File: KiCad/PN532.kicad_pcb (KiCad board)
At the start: 2 copper layers, 40 x 40 mm, 56 parts, among them J1 Bell, J2 Header, J3 SPOX, SW1 TAMPER, U1 PN532, U2 QR, U3 QR, Y1 27.12MHz

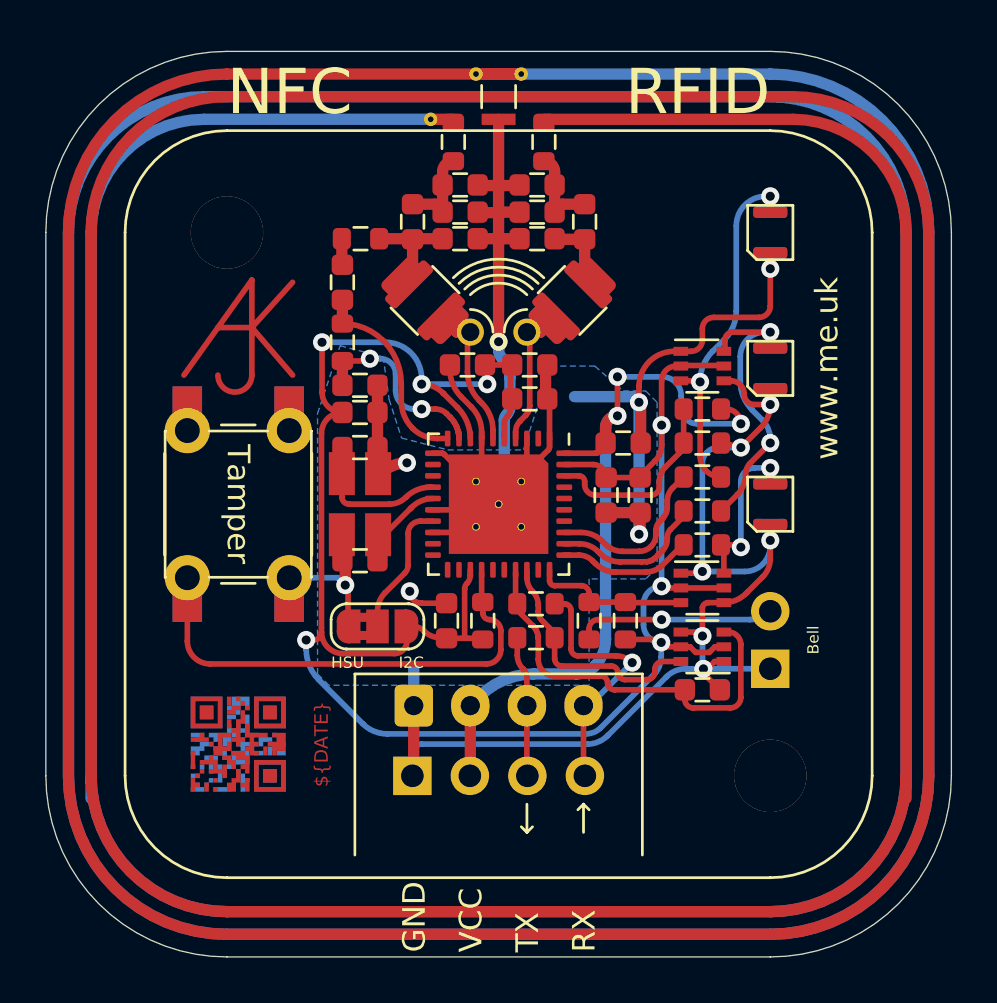
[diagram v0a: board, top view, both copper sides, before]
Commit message: Never ending tinkering
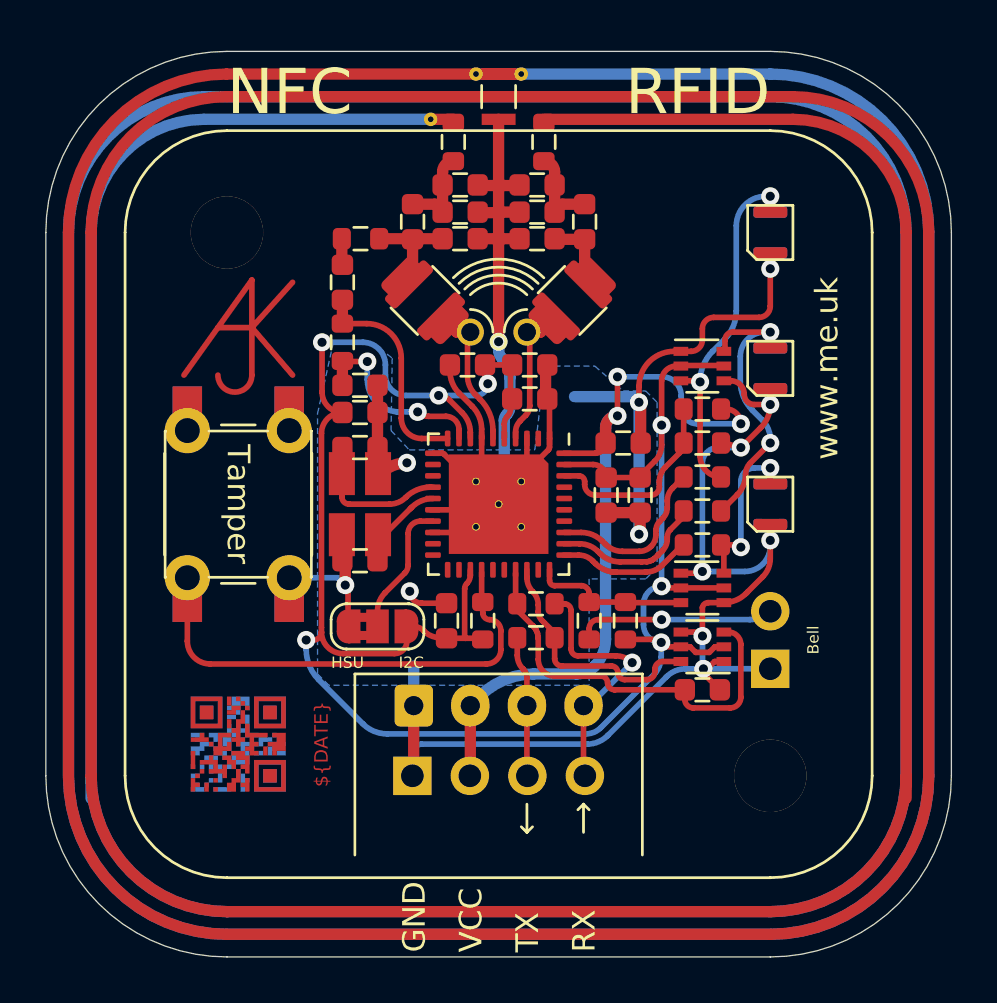
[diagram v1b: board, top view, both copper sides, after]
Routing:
- net Net-(C9-Pad1): track 9.60 -> 8.56 mm
- net Net-(C8-Pad1): track 8.91 -> 9.64 mm
